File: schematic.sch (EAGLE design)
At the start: 30 parts, among them Q1 SPB80P06P, Q2 IRF540, Q3 IRF4905

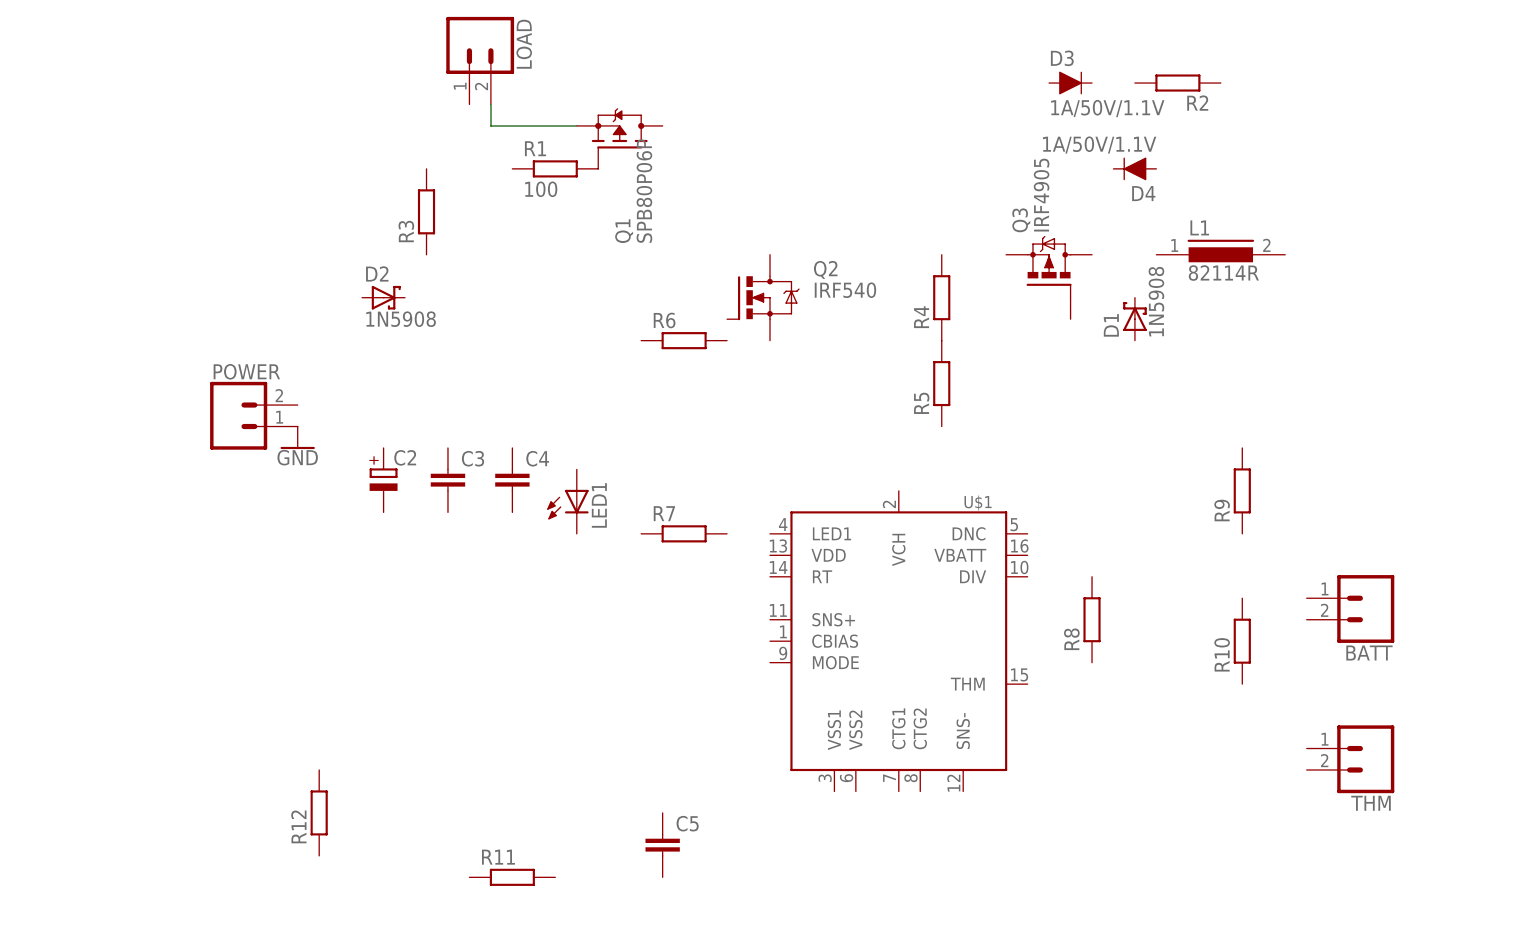
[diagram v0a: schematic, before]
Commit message: Create connections
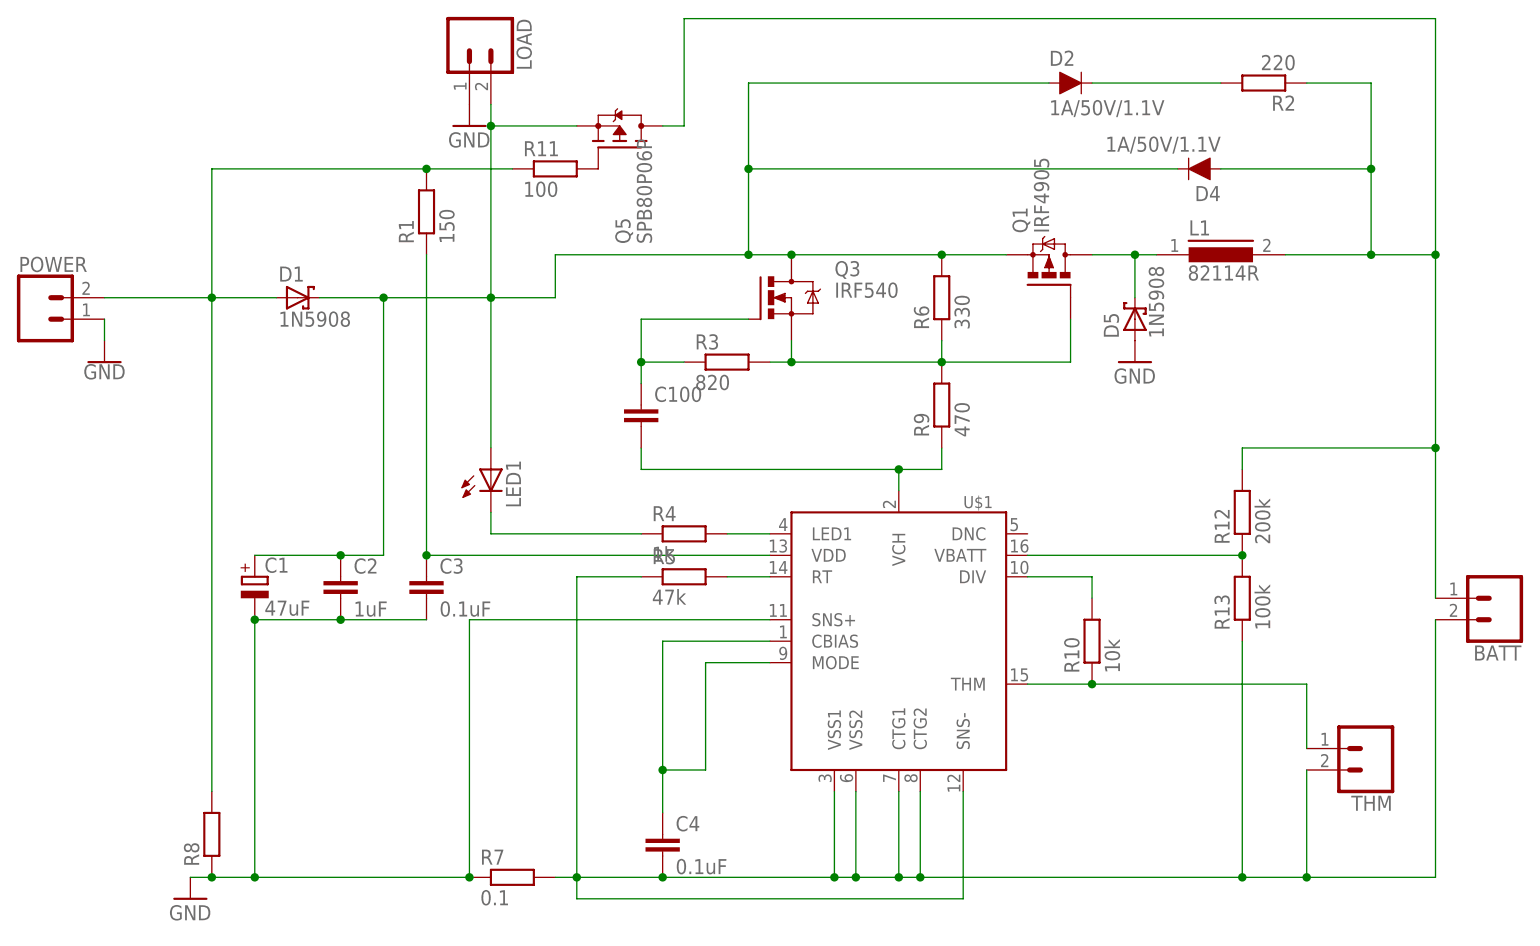
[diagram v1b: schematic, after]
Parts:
- removed C5: (no value), rcl:C-EU025-025X050
- removed D3: 1A/50V/1.1V, SparkFun-DiscreteSemi:DIODE-PTH
- removed Q2: IRF540, transistor-power:IRF540
- added C1: 47uF, rcl:CPOL-EUE2.5-6
- added C100: (no value), rcl:C-EU025-025X050
- added D5: 1N5908, diode:1N5908
- added Q5: SPB80P06P, transistor-fet:SPB80P06P
- added R13: 100k, rcl:R-EU_0207/10
- C2: value (none) -> 1uF; device rcl:CPOL-EUE2.5-6 -> rcl:C-EU025-025X050
- C3, C4: value (none) -> 0.1uF
- D2: value 1N5908 -> 1A/50V/1.1V; device diode:1N5908 -> SparkFun-DiscreteSemi:DIODE-PTH
- Q1: value SPB80P06P -> IRF4905; device transistor-fet:SPB80P06P -> transistor-power:IRF4905
- Q3: value IRF4905 -> IRF540; device transistor-power:IRF4905 -> transistor-power:IRF540
- R1: value 100 -> 150
- R10: value (none) -> 10k
- R11: value (none) -> 100
- R12: value (none) -> 200k
- R2: value (none) -> 220
- R3: value (none) -> 820
- R4: value (none) -> 1k
- R5: value (none) -> 47k
- R6: value (none) -> 330
- R7: value (none) -> 0.1
- R9: value (none) -> 470
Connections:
- removed net N$2: LOAD.2, Q1.S
- removed net N$3: R4.1, R5.2
- new net N$10: D5.C, L1.1, Q1.D
- new net N$12: C100.2, R9.1, U$1.VCH
- new net N$13: Q1.G, Q3.S, R3.2, R6.1, R9.2
- new net N$14: C100.1, Q3.G, R3.1
- new net N$15: LED1.C, R4.1
- new net N$17: D2.C, R2.2
- new net N$19: C3.1, R1.1, U$1.VDD
- new net N$20: R5.2, U$1.RT
- new net N$23: C4.1, U$1.CBIAS, U$1.MODE
- new net N$25: D1.A, POWER.2, R1.2, R11.1, R8.2
- new net N$26: C1.+, C2.1, D1.C, D2.A, D4.C, LED1.A, LOAD.2, Q1.S, Q3.D, Q5.S, R6.2
- new net N$4: BATT.2, C4.2, R13.1, R5.1, R7.2, THM.2, U$1.CTG1, U$1.CTG2, U$1.SNS-, U$1.VSS1, U$1.VSS2
- new net N$5: R10.1, THM.1, U$1.THM
- new net N$6: R10.2, U$1.DIV
- new net N$7: R12.1, R13.2, U$1.VBATT
- new net N$8: BATT.1, D4.A, L1.2, Q5.D, R12.2, R2.1
- new net N$9: R4.2, U$1.LED1
- net GND: now also C1.-, C2.2, C3.2, D5.A, LOAD.1, R7.1, R8.1, U$1.SNS+
- net N$1: now also Q5.G, R11.2; no longer Q1.G, R1.2
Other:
- moved on the sheet: BATT, C3, C4, D1, D4, LED1, POWER, R1, R10, R11, R12, R2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
